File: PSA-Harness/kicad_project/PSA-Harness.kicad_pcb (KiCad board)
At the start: 4 copper layers, 33.8 x 42.2 mm, 16 parts, among them J1 to_EPS_1, J2 to_EPS_2, J3 to_ESP_3, J4 to_car_1, J5 to_car_2, J6 to_car_3, J7 USB_C_Receptacle, U1 DG419LEUA, U2 DG419LEUA

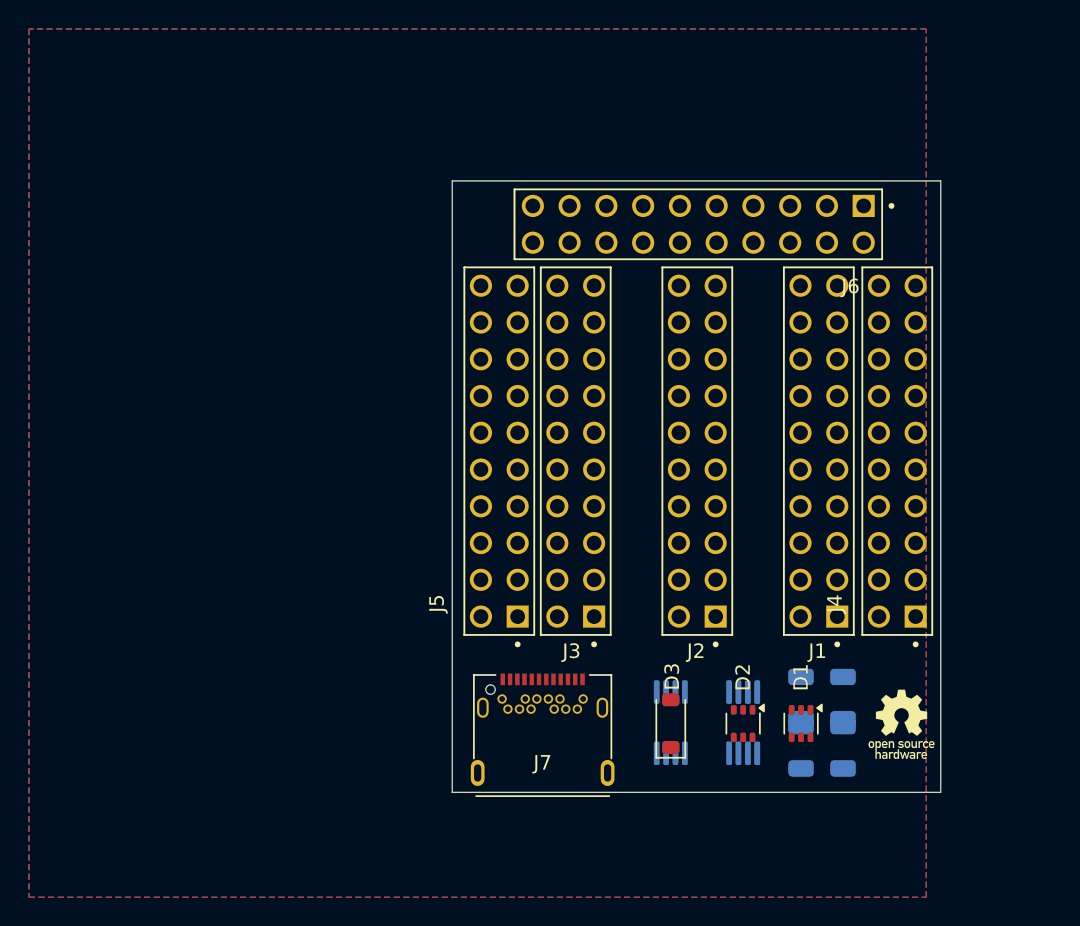
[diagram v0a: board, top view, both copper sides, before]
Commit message: components placed exactly
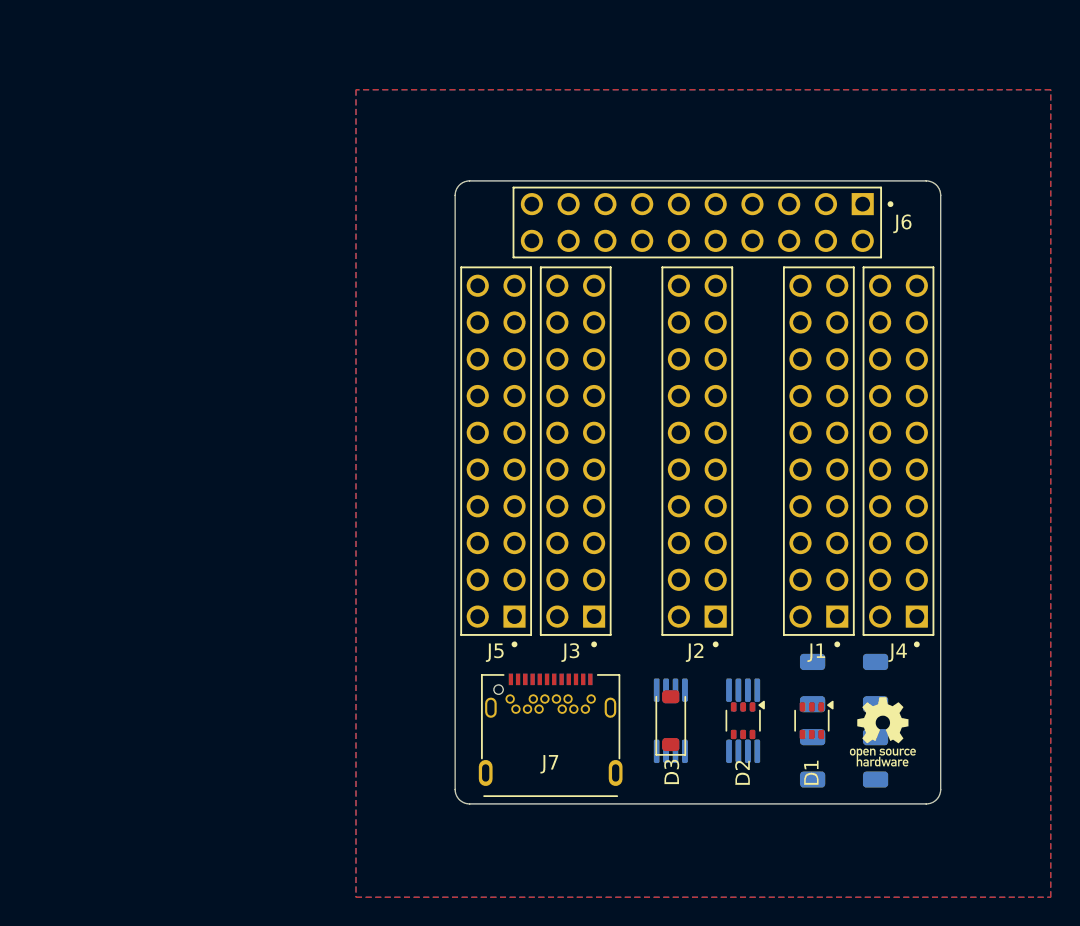
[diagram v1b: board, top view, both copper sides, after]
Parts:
- moved R3 2.48 mm to (118.0, 138.2)
- moved R4 2.38 mm to (118.0, 143.4)
- moved R2 1.31 mm to (113.7, 138.2)
- moved R1 1.11 mm to (113.7, 143.4)
- moved D1 0.78 mm to (113.6, 140.8)
- moved J7 0.55 mm to (95.5, 143.0)
- moved J5 0.22 mm to (91.8, 122.2)
- moved D2 0.20 mm to (108.8, 140.8)
- moved D3 0.20 mm to (103.8, 140.8)
- moved J6 0.14 mm to (105.7, 106.4)
- moved U1 0.14 mm to (103.8, 140.8)
- moved U2 0.14 mm to (108.8, 140.8)
- moved J4 0.08 mm to (119.6, 122.2)
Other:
- board size 33.8 x 42.2 mm -> 33.5 x 43.1 mm
